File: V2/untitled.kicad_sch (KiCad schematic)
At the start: 28 parts

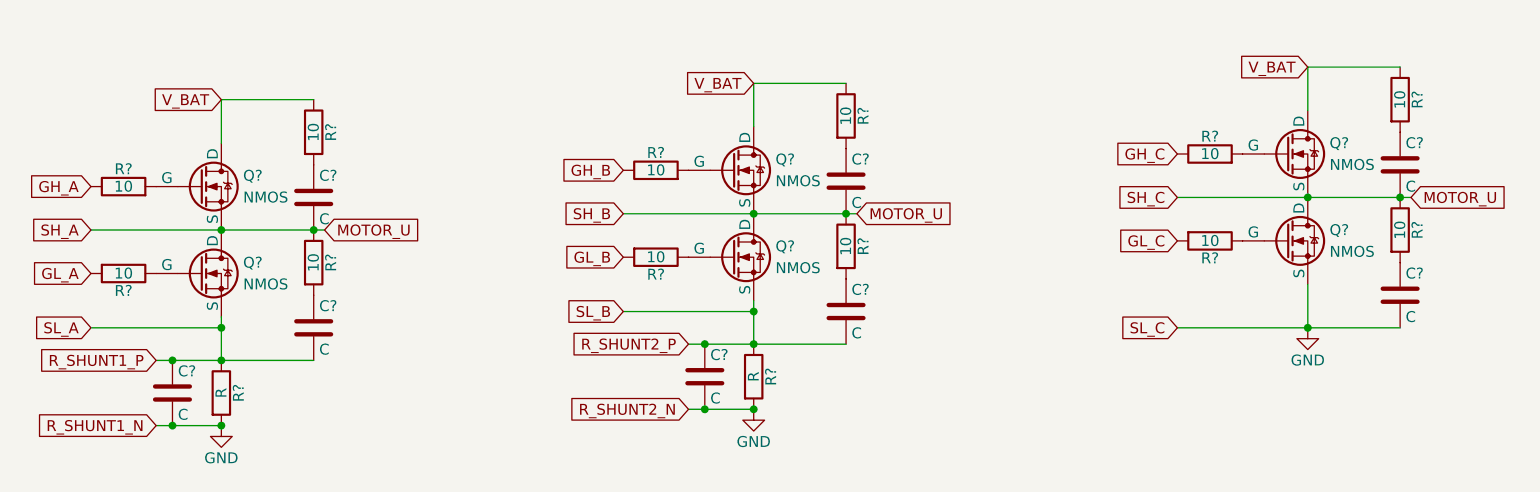
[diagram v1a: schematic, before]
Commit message: def
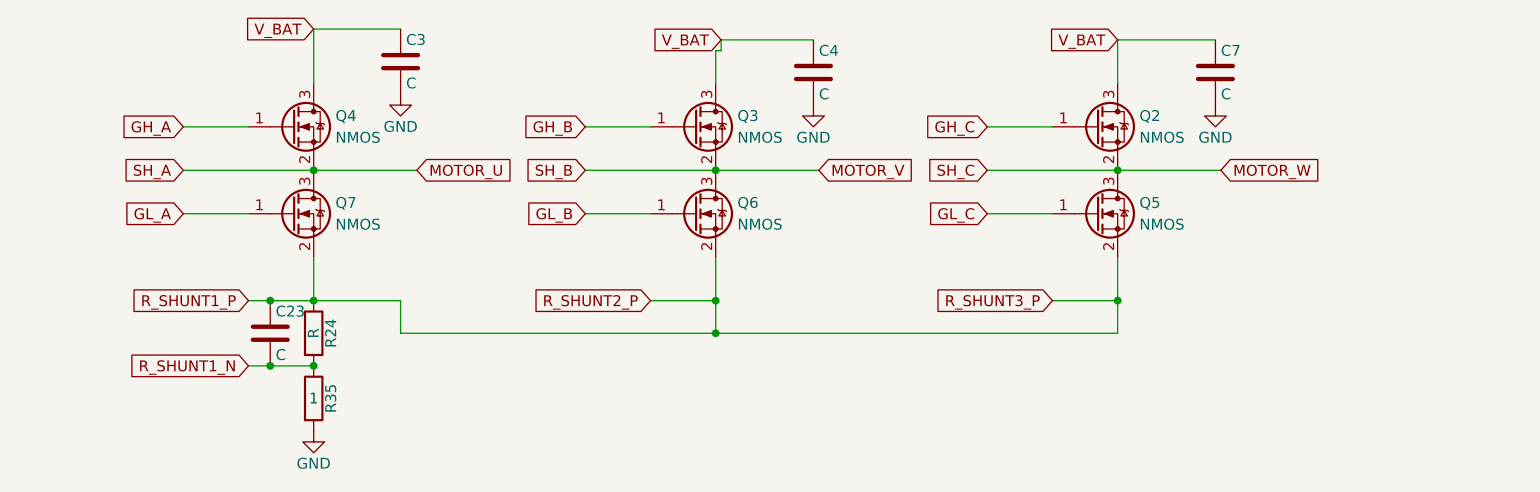
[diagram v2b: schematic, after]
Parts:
- removed C? (x7): C, Capacitor_SMD:C_0201_0603Metric, symbol Device:C
- removed R? (x12): 10, Resistor_SMD:R_1206_3216Metric, symbol Device:R
- removed R?: R, Resistor_SMD:R_1206_3216Metric, symbol Device:R
- added C3, C4, C7: C, Dam_libkicad:0603, symbol Device:C
- added R35: 1, Dam_libkicad:0603, symbol Device:R
- C23: renamed from C?; footprint Capacitor_SMD:C_0201_0603Metric -> Dam_libkicad:0603
- Q2, Q3, Q4, Q5, Q6, Q7: renamed from Q?; footprint Package_TO_SOT_SMD:SOT-23 -> Package_TO_SOT_SMD:TO-263-2; symbol Simulation_SPICE:NMOS -> Device:Q_NMOS_GSD
- R24: renamed from R?; footprint Resistor_SMD:R_1206_3216Metric -> Dam_libkicad:0603
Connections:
- net R_SHUNT2_P is gone; now on net MOTOR_V: Q6.3 (D)
- net GH_A: now also Q4.1 (G)
- net GH_B: now also Q3.1 (G)
- net GH_C: now also Q2.1 (G)
- net GL_A: now also Q7.1 (G)
- net GL_B: now also Q6.1 (G)
- net GL_C: now also Q5.1 (G)
- net GND: now also C3.2, C4.2, C7.2, R35.2; no longer C23.2, Q5.3 (S), R24.2
- net MOTOR_U: now also Q4.2 (S), Q7.3 (D); no longer Q2.3 (S), Q3.3 (S), Q4.3 (S), Q5.1 (D), Q6.1 (D), Q7.1 (D)
- net R_SHUNT1_P: now also Q5.2 (S), Q6.2 (S), Q7.2 (S); no longer Q7.3 (S)
- net V_BAT: now also Q2.3 (D), Q3.3 (D), Q4.3 (D), C3.1, C4.1, C7.1; no longer Q2.1 (D), Q3.1 (D), Q4.1 (D)
- net MOTOR_V: now reaches Q3.2 (S)
- net MOTOR_W: now reaches Q2.2 (S)
- net MOTOR_W: now also Q5.3 (D)
- new net R_SHUNT1_N: C23.2, R24.2, R35.1
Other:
- moved on the sheet: C23, Q2, Q3, Q4, Q5, Q6, Q7, R24
